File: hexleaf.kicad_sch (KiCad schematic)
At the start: 42 parts, among them IC1 ESP32-C3-FH4, J2 Conn_01x04, J5 Conn_01x08, J6 Conn_01x04, J7 Conn_01x08, SW1 SW_SPST, SW2 SW_SPST, Y1 ECS-400-10-37B2-CKM-TR

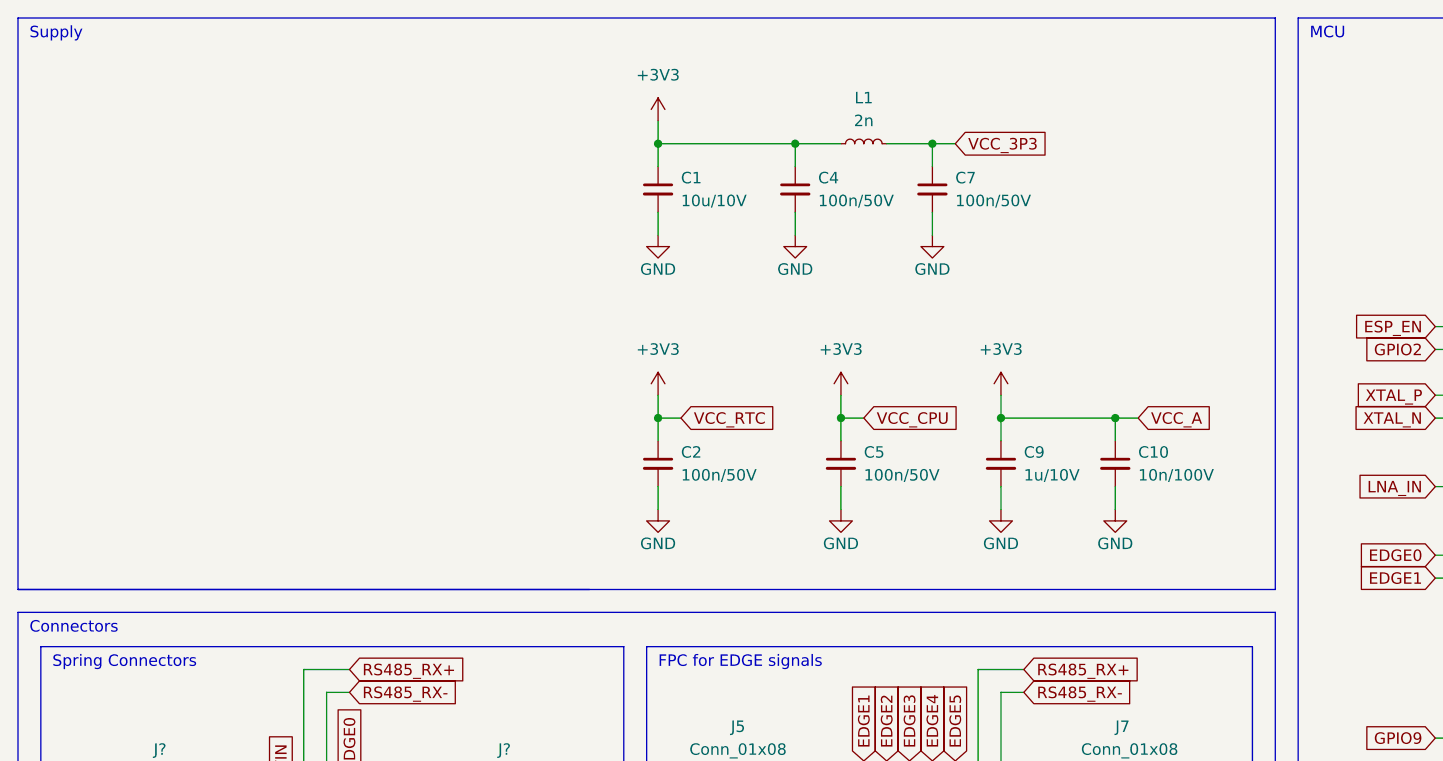
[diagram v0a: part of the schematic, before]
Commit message: added buck
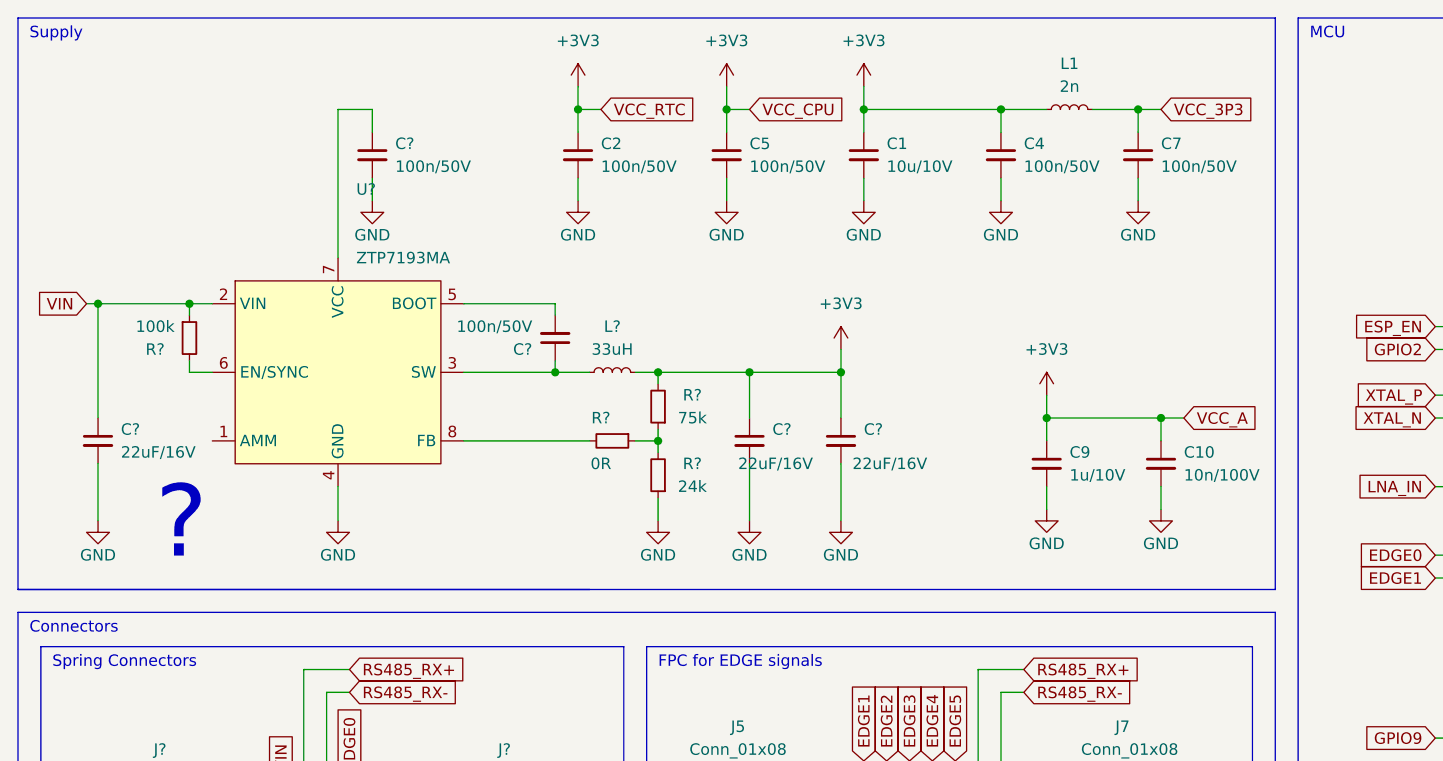
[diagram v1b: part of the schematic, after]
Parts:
- added C? (x3): 22uF/16V, Resistor_SMD:R_0603_1608Metric, symbol Device:C_Small
- added C? (x2): 100n/50V, Resistor_SMD:R_0603_1608Metric, symbol Device:C_Small
- added L?: 33uH, hexleaf:CYH127, symbol Device:L_Small
- added R?: 24k, Resistor_SMD:R_0603_1608Metric, symbol Device:R_Small
- added R?: 75k, Resistor_SMD:R_0603_1608Metric, symbol Device:R_Small
- added R?: 100k, Resistor_SMD:R_0603_1608Metric, symbol Device:R_Small
- added R?: 0R, Resistor_SMD:R_0603_1608Metric, symbol Device:R_Small
- added U?: ZTP7193MA, Package_TO_SOT_SMD:SOT-23-8, symbol hexleaf:ZTP7193MA
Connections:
- net +3V3: now also C?.1, C?.1, L?.2, R?.2
- net GND: now also C?.2, C?.2, C?.2, C?.2, R?.1, U?.4 (GND)
- net VIN: now also C?.1, R?.1, U?.2 (VIN)
- new net: C?.1, L?.1, U?.3 (SW)
- new net: C?.2, U?.5 (BOOT)
- new net: R?.2, U?.6 (EN/SYNC)
- new net: C?.1, U?.7 (VCC)
- new net: R?.2, U?.8 (FB)
- new net: R?.1, R?.1, R?.2
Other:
- note added: "?"
- moved on the sheet: C1, C10, C2, C4, C5, C7, C9, L1
